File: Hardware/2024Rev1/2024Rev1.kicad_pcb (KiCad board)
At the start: 2 copper layers, 116.6 x 93.7 mm, 86 parts, among them J7 RJ45_LED_Shielded, Q2 BSS138, Q3 BSS138, Q5 BSS138, Q6 SPD30P06PGBTMA1, Q7 BSS138, U2 Opamp_Dual, U3 Teensy4.1_DEV-16771, U4 Opamp_Dual, U5 Opamp_Dual, U6 Opamp_Dual, U7 ACS758xCB-200B-PFF, U8 OKI, U9 OKI

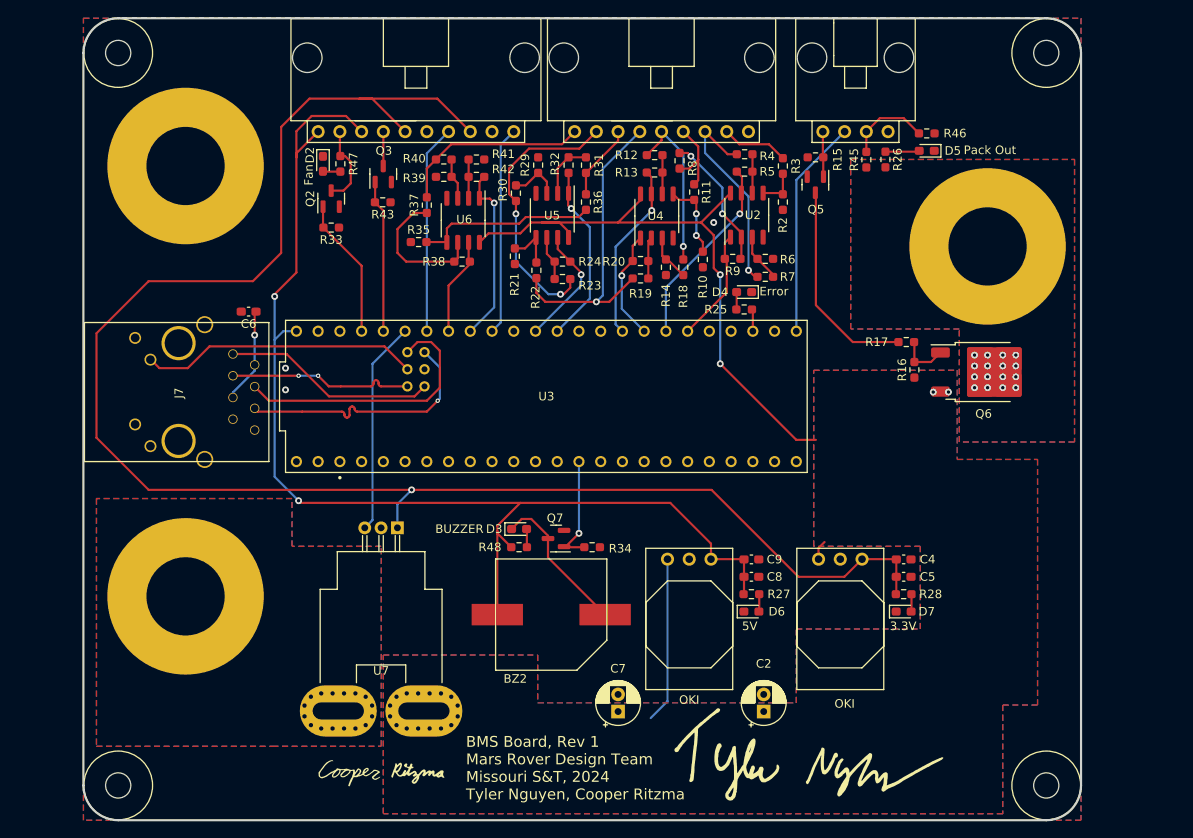
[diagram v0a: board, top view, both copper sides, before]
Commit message: rearranged components and flags. also started on some traces
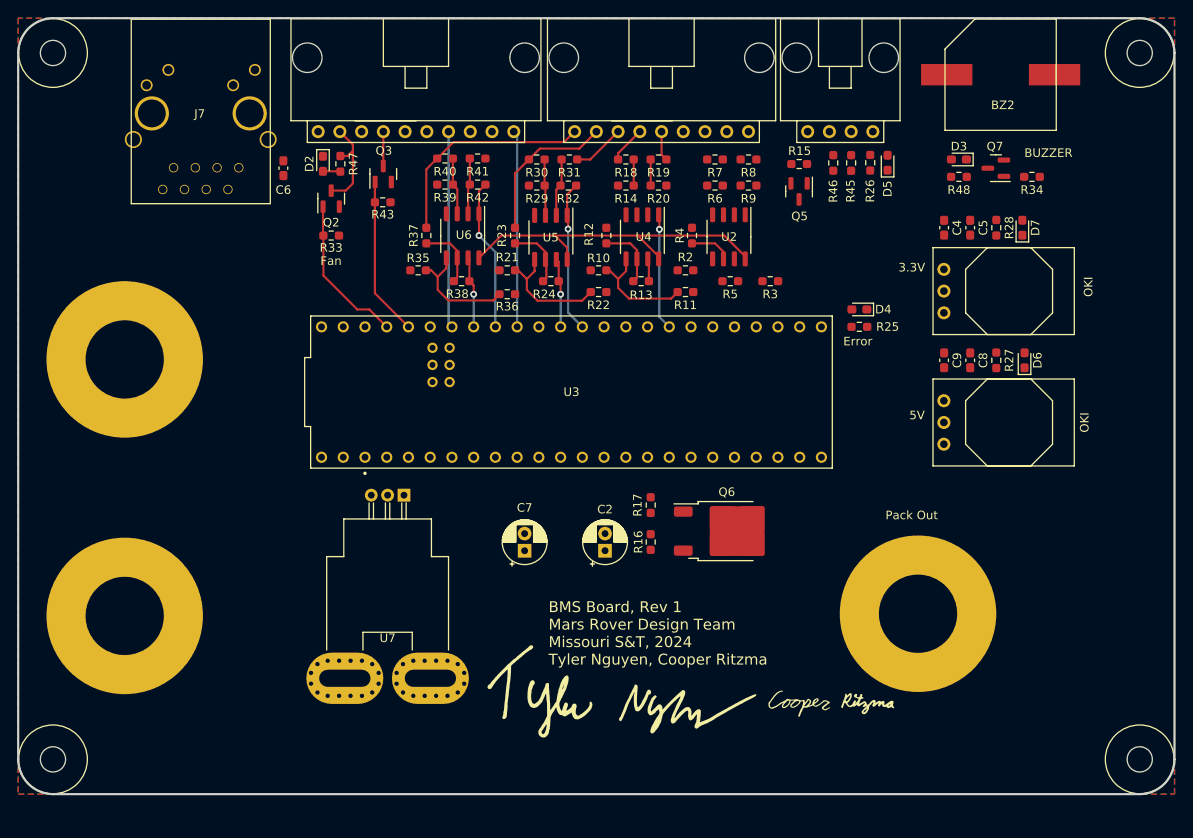
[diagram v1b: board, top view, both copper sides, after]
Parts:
- moved BZ2 91.0 mm to (216.6, 43.4), turned to 180 degrees
- moved R34 67.2 mm to (213.7, 55.4)
- moved R48 67.2 mm to (205.2, 55.4), turned to 0 degrees
- moved Q7 67.2 mm to (209.5, 54.4)
- moved D3 67.1 mm to (205.2, 53.3), turned to 180 degrees
- moved G*** 53.2 mm to (190.2, 116.8)
- moved J7 48.2 mm to (116.5, 35.0), turned to 180 degrees
- moved D7 47.0 mm to (212.6, 61.3), turned to 90 degrees
- moved R28 44.2 mm to (209.6, 61.3), turned to -90 degrees
- moved V4 43.7 mm to (200.4, 106.4)
- moved D6 43.4 mm to (212.9, 76.8), turned to 90 degrees
- moved C5 41.5 mm to (206.5, 61.3), turned to 90 degrees
- moved R27 39.6 mm to (209.6, 76.8), turned to -90 degrees
- moved C4 39.0 mm to (203.5, 61.3), turned to 90 degrees
- moved R16 36.8 mm to (169.2, 98.0)
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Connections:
- Conn3 pad 4: cell4 -> cell5
- Conn3 pad 5: cell5 -> cell4
- Conn3 pad 6: cell6 -> cell7
- Conn3 pad 7: cell7 -> cell6
- U3 pad 12: Buzzer-Teensy -> unconnected-(U3-MISO-Pad12)
- U3 pad 21: CURRENT_SENSE -> unconnected-(U3-A7-Pad21)
- U3 pad 24: unconnected-(U3-A10-Pad24) -> CURRENT_SENSE
- U3 pad 33: GATE -> ERR_LED
- U3 pad 34: unconnected-(U3-RX8-Pad34) -> Buzzer-Teensy
- U3 pad 35: ERR_LED -> GATE
- U3 pad R-: R- -> (no net)
- U3 pad T-: T- -> (no net)
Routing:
- net +3.3V: track 194.7 -> 0.00 mm, vias 1 -> 0
- net +5V: track 138.3 -> 0.00 mm, vias 2 -> 0
- net PackLogic: track 94.3 -> 40.6 mm, vias 4 -> 0
- net cell4: track 36.5 -> 3.49 mm, vias 1 -> 0
- net LED: track 32.6 -> 0.00 mm
- net R+: track 32.0 -> 0.00 mm
- net R-: track 30.5 -> 0.00 mm, vias 1 -> 0
- net GATE: track 25.7 -> 0.00 mm
- net CURRENT_SENSE: track 24.9 -> 0.00 mm
- net T+: track 24.9 -> 0.00 mm
- net Net-(Q5-D): track 24.6 -> 0.00 mm
- net cell7: track 24.5 -> 0.00 mm, vias 1 -> 0
- net Cell8-SENSE: track 22.6 -> 0.00 mm, vias 1 -> 0
- net T-: track 21.8 -> 0.00 mm, vias 2 -> 0
- net Cell6-SENSE: track 20.9 -> 2.66 mm, vias 1 -> 0
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- removed copper zone on B.Cu, net Net-(U7-IP+)
- removed copper zone on F.Cu, net Net-(U7-IP+)
- removed copper zone on B.Cu, net PACK_OUT
- removed copper zone on F.Cu, net PACK_OUT
- removed copper zone on B.Cu, net PackLogic
- removed copper zone on F.Cu, net PackLogic
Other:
- board size 116.6 x 93.7 mm -> 135.1 x 90.7 mm
